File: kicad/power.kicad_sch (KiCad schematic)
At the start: 28 parts, among them J2 POWER_IN, J5 Conn_01x04, J7 Barrel_Jack_Switch, U10 40106, U2 LM358

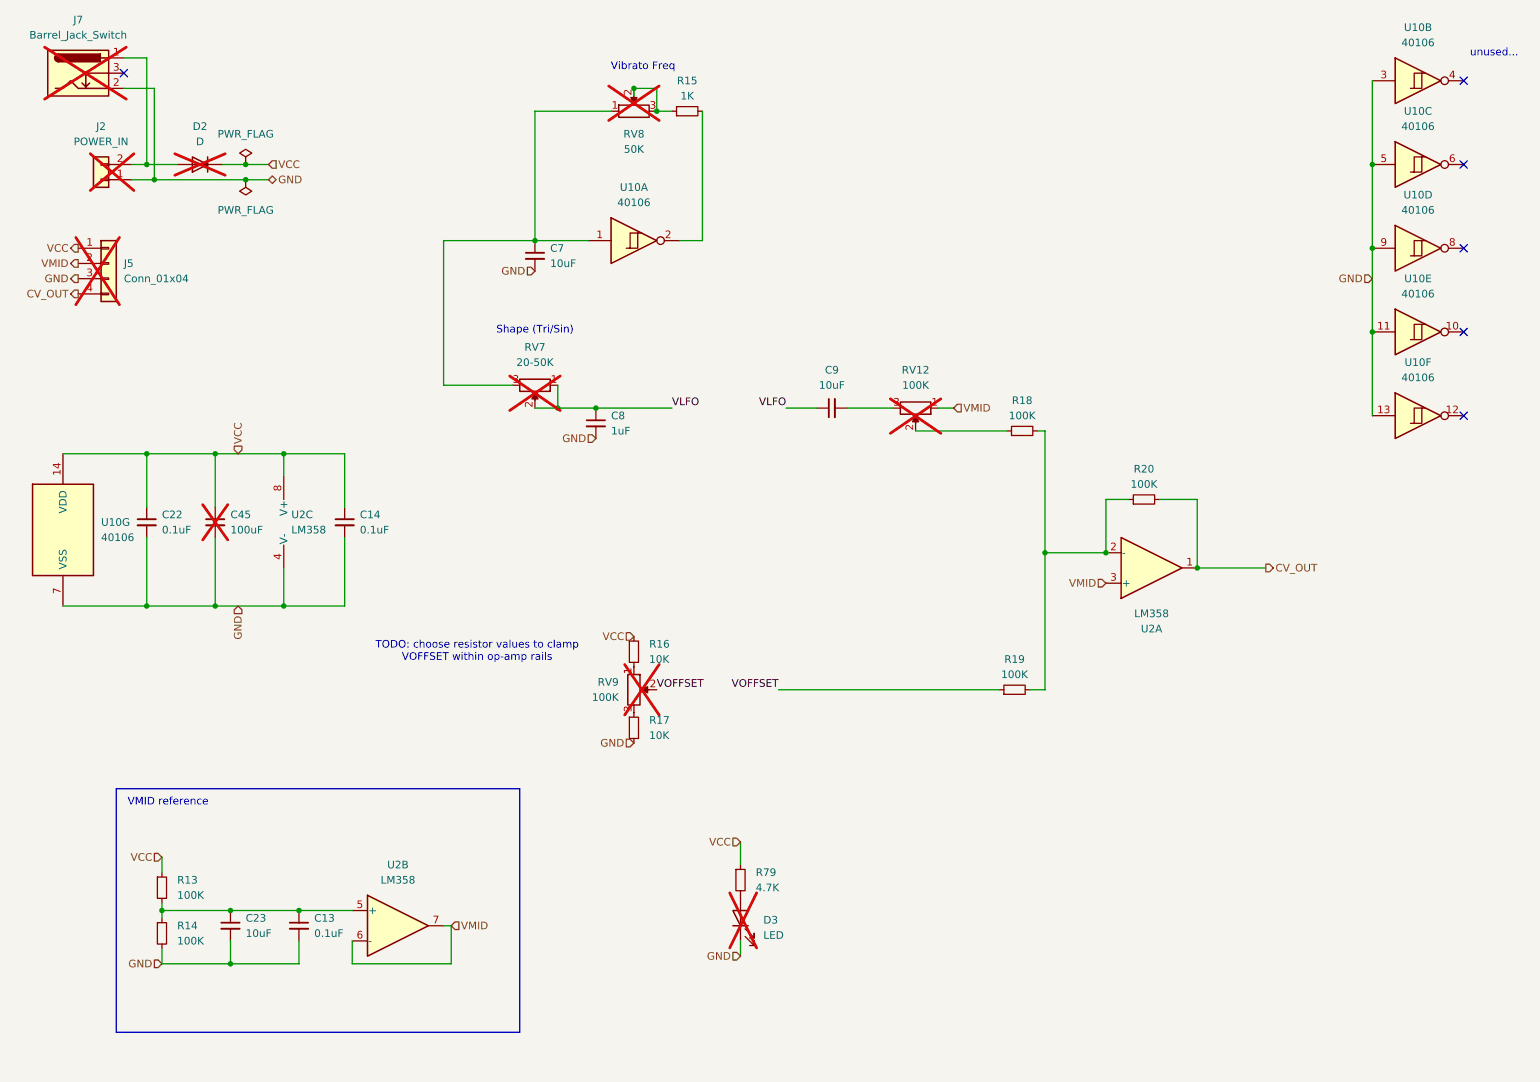
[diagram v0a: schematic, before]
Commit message: add local changes
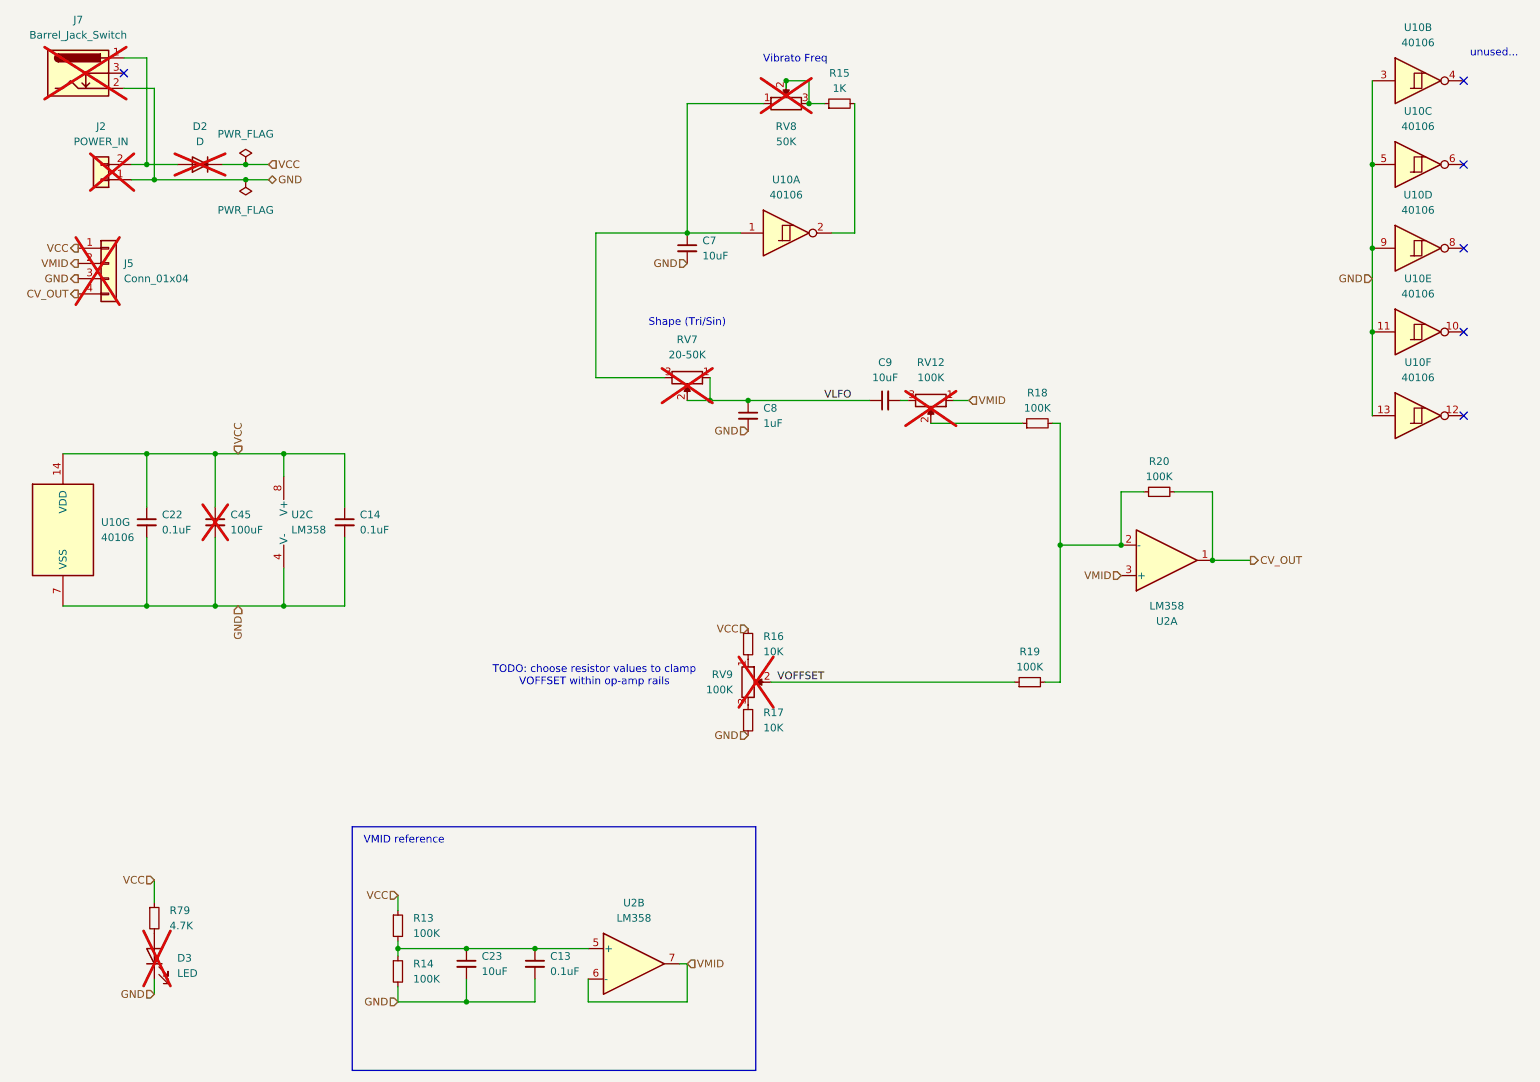
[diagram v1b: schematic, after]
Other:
- moved on the sheet: C13, C23, C7, C8, C9, D3, R13, R14, R15, R16, R17, R18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
